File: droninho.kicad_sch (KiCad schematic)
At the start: 19 parts, among them J1 Conn_01x02_Pin, J2 M2, J3 M1, J4 M3, J5 M4, Q1 SI2300, Q2 SI2300, Q3 SI2300, Q4 SI2300, U1 ESP32 Dev Kit, U3 MPU9250/6500

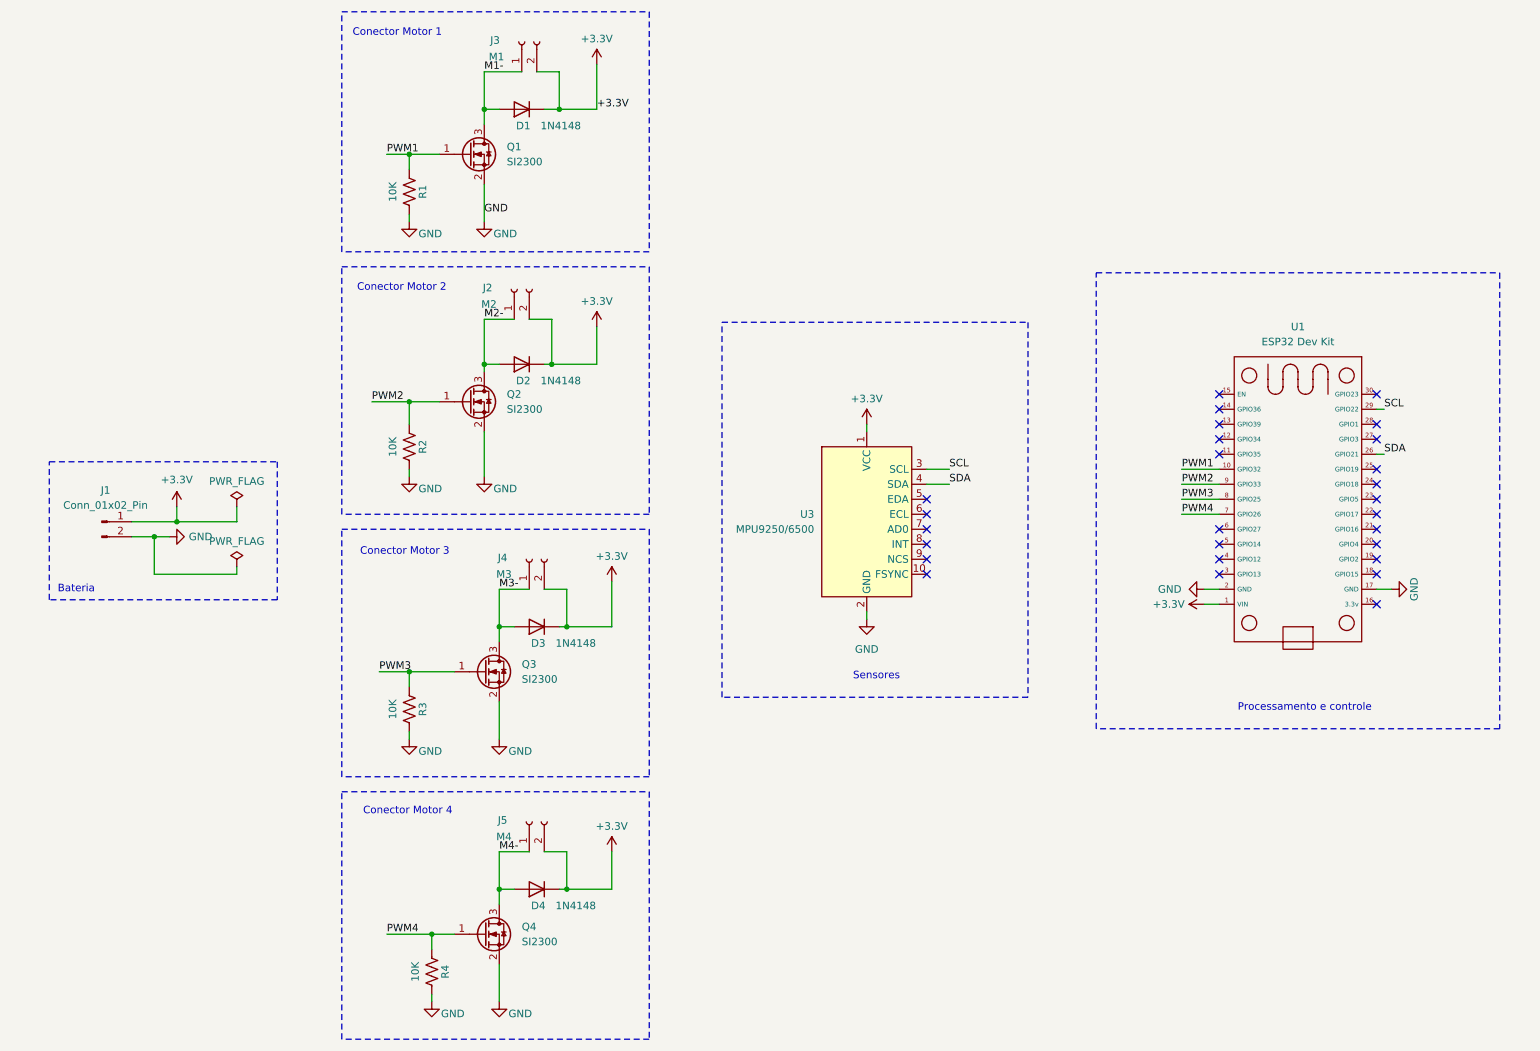
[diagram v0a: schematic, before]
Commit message: PCB finalizado.
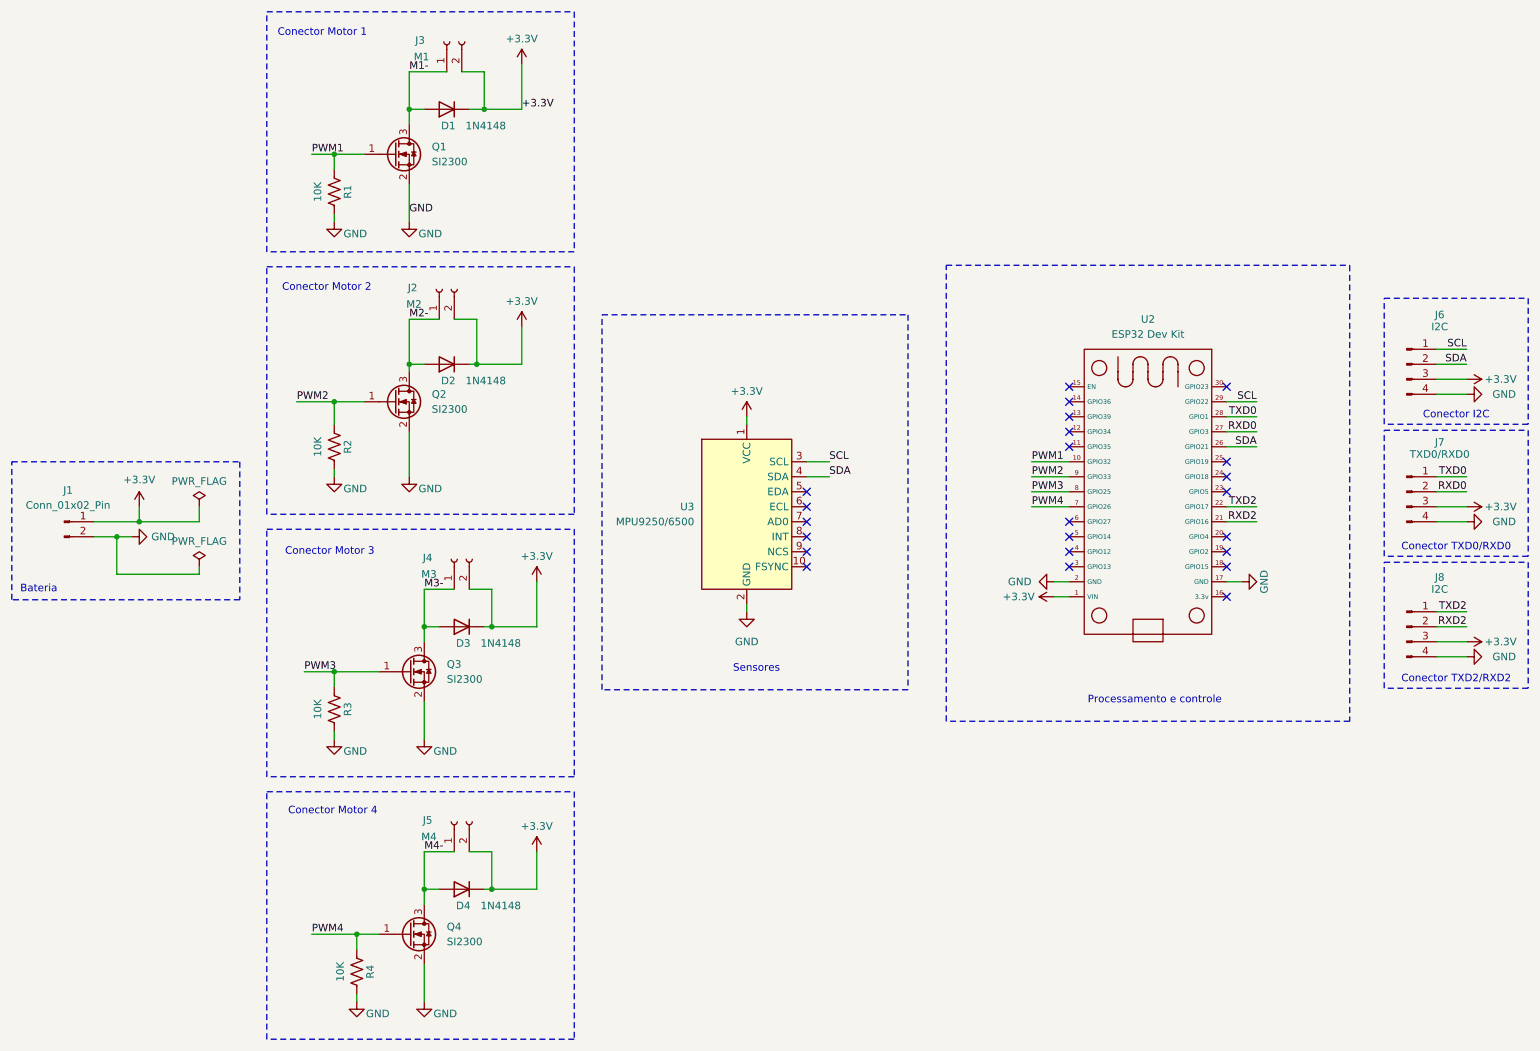
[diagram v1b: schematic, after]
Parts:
- removed U1: ESP32 Dev Kit, Library:ESP32_30pin, symbol Library:ESP32_30Pin
- added J6, J8: I2C, Connector:FanPinHeader_1x04_P2.54mm_Vertical, symbol Connector:Conn_01x04_Pin
- added J7: TXD0/RXD0, Connector:FanPinHeader_1x04_P2.54mm_Vertical, symbol Connector:Conn_01x04_Pin
- added U2: ESP32 Dev Kit, Library:ESP32_30pin, symbol Library:ESP32_30Pin
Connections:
- net +3.3V: now also J6.3 (Pin_3), J7.3 (Pin_3), J8.3 (Pin_3), U2.1 (VIN)
- net GND: now also J6.4 (Pin_4), J7.4 (Pin_4), J8.4 (Pin_4), U2.17 (GND), U2.2 (GND)
- net PWM1: now also U2.10 (GPIO32)
- net PWM2: now also U2.9 (GPIO33)
- net PWM3: now also U2.8 (GPIO25)
- net PWM4: now also U2.7 (GPIO26)
- net SCL: now also J6.1 (Pin_1), U2.29 (GPIO22)
- net SDA: now also J6.2 (Pin_2), U2.26 (GPIO21)
- new net RXD0: J7.2 (Pin_2), U2.27 (GPIO3)
- new net RXD2: J8.2 (Pin_2), U2.21 (GPIO16)
- new net TXD0: J7.1 (Pin_1), U2.28 (GPIO1)
- new net TXD2: J8.1 (Pin_1), U2.22 (GPIO17)
- no-connect marks 27 -> 23
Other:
- note added: "Conector I2C"
- note added: "Conector TXD0/RXD0"
- note added: "Conector TXD2/RXD2"
- moved on the sheet: D1, D2, D3, D4, J1, J2, J3, J4, J5, Q1, Q2, Q3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
